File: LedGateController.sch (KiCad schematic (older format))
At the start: 48 parts, among them J1 5050_OUT, J2 SWD, J3 GPIO, Q1 FS8205A, Q2 AO3400A, Q3 AO3400A, Q4 AO3400A, SW1 SW_SPST, SW2 BUTTON, U1 AP2127N-3.3, U2 MT3608, U3 DW01, U4 STM32F030F4Px

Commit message: Move to footprints
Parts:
- removed Q3, Q4: AO3400A, Package_TO_SOT_SMD:SOT-23, symbol MiscParts:AO3400A
- removed R11, R12, R13: 100, Resistor_SMD:R_0805_2012Metric_Pad1.15x1.40mm_HandSolder, symbol Device:R
- removed TP3: +3V3, TestPoint:TestPoint_THTPad_2.0x2.0mm_Drill1.0mm, symbol Connector:TestPoint
- removed TP4: +12V, TestPoint:TestPoint_THTPad_2.0x2.0mm_Drill1.0mm, symbol Connector:TestPoint
- removed TP7: NRST, TestPoint:TestPoint_THTPad_2.0x2.0mm_Drill1.0mm, symbol Connector:TestPoint
- removed U1: AP2127N-3.3, Package_TO_SOT_SMD:SOT-23, symbol Regulator_Linear:AP2127N-3.3
- added C12, C14: 100n, Capacitor_SMD:C_0805_2012Metric_Pad1.15x1.40mm_HandSolder, symbol Device:C
- added C13: 470u, Capacitor_SMD:CP_Elec_10x7.7, symbol Device:CP
- added Q3: AO3401A, Package_TO_SOT_SMD:SOT-23, symbol Transistor_FET:AO3401A
- added R6, R7: 100, Resistor_SMD:R_0805_2012Metric_Pad1.15x1.40mm_HandSolder, symbol Device:R
- added TP5: LED_DATA_3V3, TestPoint:TestPoint_THTPad_D2.0mm_Drill1.0mm, symbol Connector:TestPoint
- added TP6: LED_DATA_5V, TestPoint:TestPoint_THTPad_D2.0mm_Drill1.0mm, symbol Connector:TestPoint
- added U4: XC6206P332MR, Package_TO_SOT_SMD:SOT-23, symbol Regulator_Linear:XC6206PxxxMR
- added U5: PI4ULS5V201, Package_TO_SOT_SMD:SOT-23-6_Handsoldering, symbol MiscParts:PI4ULS5V201
- BT1: value 18650 -> LI_ON; Digikey Part (none) -> https://www.digikey.co.uk/product-detail/en/keystone-electr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
- C1: renamed from C9; value 100nF -> 100n; footprint (none) -> Capacitor_SMD:C_0805_2012Metric_Pad1.15x1.40mm_HandSolder; LCSC Part (none) -> https://lcsc.com/product-detail/Multilayer-Ceramic-Capacito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
- C10: renamed from C1; value 0.1uF -> 1u; LCSC Part (none) -> https://lcsc.com/product-detail/Multilayer-Ceramic-Capacito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
- C11: renamed from C4; value 0.1uF -> 1u; LCSC Part (none) -> https://lcsc.com/product-detail/Multilayer-Ceramic-Capacito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
- C2: value 22uF -> 22u; footprint (none) -> Capacitor_SMD:C_0805_2012Metric_Pad1.15x1.40mm_HandSolder; LCSC Part (none) -> https://lcsc.com/product-detail/Multilayer-Ceramic-Capacito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
- C3: renamed from C6; value 100nF -> 100n; footprint (none) -> Capacitor_SMD:C_0805_2012Metric_Pad1.15x1.40mm_HandSolder; LCSC Part (none) -> https://lcsc.com/product-detail/Multilayer-Ceramic-Capacito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
- C4: renamed from C10; value 100nF -> 100n; footprint (none) -> Capacitor_SMD:C_0805_2012Metric_Pad1.15x1.40mm_HandSolder; LCSC Part (none) -> https://lcsc.com/product-detail/Multilayer-Ceramic-Capacito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
- C5: renamed from C3; value 0.1uF -> 100n; LCSC Part (none) -> https://lcsc.com/product-detail/Multilayer-Ceramic-Capacito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
- C6: renamed from C11; value 4.7uF -> 4u7; footprint (none) -> Capacitor_SMD:C_0805_2012Metric_Pad1.15x1.40mm_HandSolder; LCSC Part (none) -> https://lcsc.com/product-detail/Multilayer-Ceramic-Capacito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
- C7: renamed from C12; value 1uF -> 1u; footprint (none) -> Capacitor_SMD:C_0805_2012Metric_Pad1.15x1.40mm_HandSolder
- C8: renamed from C13; value 10nF -> 10n; footprint (none) -> Capacitor_SMD:C_0805_2012Metric_Pad1.15x1.40mm_HandSolder; LCSC Part (none) -> https://lcsc.com/product-detail/Multilayer-Ceramic-Capacito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
- C9: renamed from C5; value 22uF -> 22u; footprint (none) -> Capacitor_SMD:C_0805_2012Metric_Pad1.15x1.40mm_HandSolder; LCSC Part (none) -> https://lcsc.com/product-detail/Multilayer-Ceramic-Capacito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
- D1: value D_Schottky -> SS22; footprint (none) -> Diode_SMD:D_SMA_Handsoldering; LCSC Part (none) -> https://lcsc.com/product-detail/Schottky-Barrier-Diodes-SBD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
- D2: footprint (none) -> LED_SMD:LED_0805_2012Metric_Pad1.12x1.40mm_HandSolder; LCSC Part (none) -> https://jlcpcb.com/parts/componentSearch?secondSortUuid=ac4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
- J1: renamed from J3; footprint (none) -> Connector_PinHeader_2.54mm:PinHeader_1x10_P2.54mm_Vertical
- J2: footprint (none) -> Connector_PinHeader_2.54mm:PinHeader_1x05_P2.54mm_Vertical; symbol Connector:Conn_01x04_Male -> Connector:Conn_01x05_Male
- J3: renamed from J1; value 5050_OUT -> LED_OUT; footprint (none) -> Connector_PinHeader_2.54mm:PinHeader_1x03_P2.54mm_Horizontal; symbol Connector:Conn_01x04_Male -> Connector:Conn_01x03_Male
- L1: value 22uH -> 22u; footprint (none) -> Inductor_SMD:L_10.4x10.4_H4.8; LCSC Part (none) -> https://lcsc.com/product-detail/Power-Inductors_TDG-TMAX-10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
- Q1: footprint SOP65P640X120-8N -> Package_SO:TSSOP-8_4.4x3mm_P0.65mm; LCSC Part (none) -> https://lcsc.com/product-detail/MOSFET_Fortune-Semicon-FS82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
- Q2: LCSC Part (none) -> https://lcsc.com/product-detail/MOSFET_UMW-Youtai-Semicondu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
- R1: value 100R -> 100; LCSC Part (none) -> https://lcsc.com/product-detail/Chip-Resistor-Surface-Mount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
- R10: renamed from R9; value 33k -> 100K; LCSC Part (none) -> https://lcsc.com/product-detail/Chip-Resistor-Surface-Mount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
- R2: renamed from R6; value 100k -> 100K; LCSC Part (none) -> https://lcsc.com/product-detail/Chip-Resistor-Surface-Mount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
- R3: renamed from R2; value 5.6k -> 15K; LCSC Part (none) -> https://lcsc.com/product-detail/Chip-Resistor-Surface-Mount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
- R4: renamed from R3; value 100k -> 110K; LCSC Part (none) -> https://lcsc.com/product-detail/Chip-Resistor-Surface-Mount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
- R5: renamed from R4; value 1kR -> 1K; LCSC Part (none) -> https://lcsc.com/product-detail/Chip-Resistor-Surface-Mount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
- R8: renamed from R5; value 330R -> 150; LCSC Part (none) -> https://lcsc.com/product-detail/Chip-Resistor-Surface-Mount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
- R9: renamed from R8; value 100k -> 50K; LCSC Part (none) -> https://lcsc.com/product-detail/Chip-Resistor-Surface-Mount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
- SW1: renamed from SW2; footprint (none) -> Button_Switch_THT:SW_PUSH_6mm; LCSC Part (none) -> https://lcsc.com/product-detail/Tactile-Switches_SHOU-HAN-T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
- SW2: renamed from SW1; value SW_SPST -> ON_OFF; footprint (none) -> Button_Switch_THT:SW_CuK_OS102011MA1QN1_SPDT_Angled; symbol Switch:SW_SPST -> Switch:SW_SPDT; LCSC Part (none) -> https://lcsc.com/product-detail/Toggle-Switches_C-K_OS10201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
- TP2: footprint TestPoint:TestPoint_THTPad_2.0x2.0mm_Drill1.0mm -> TestPoint:TestPoint_THTPad_D2.0mm_Drill1.0mm
- TP3: renamed from TP8; value 12V_FB -> 5V_FB; footprint TestPoint:TestPoint_THTPad_2.0x2.0mm_Drill1.0mm -> TestPoint:TestPoint_THTPad_D2.0mm_Drill1.0mm
- U1: renamed from U4; LCSC Part (none) -> https://lcsc.com/product-detail/Others_STMicroelectronics_S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
- U2: footprint SOT95P280X145-6N -> Package_TO_SOT_SMD:SOT-23-6_Handsoldering; LCSC Part (none) -> https://lcsc.com/product-detail/DC-DC-Converters_MT3608_C84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
- U3: footprint SOT95P280X135-6N -> Package_TO_SOT_SMD:SOT-23-6_Handsoldering; LCSC Part (none) -> https://lcsc.com/product-detail/MOSFET_DW01_C181096.html; Manufacturer_Name Slkor -> (none)
- renumbered TP6 to TP4, TP5 to TP7
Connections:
- net labels added: +5V, +BATT_SW, LED_DATA_3V3, LED_DATA_5V, LED_EN, NRST, PA6, PA7
- net labels removed: +12V, -BATT, B, G, PA2, PA9, R
- wire segments 138 -> 177
- no-connect marks 5 -> 4
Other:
- note added: "Battery Switch"
- note added: "LED Logic Shifter"
- note added: "LED Supply (5V)"
- note removed: "LED Supply (12V)"
- moved on the sheet: C1, C10, C11, C2, C3, C4, C5, C6, C7, C8, C9, D1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

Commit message: nearly done
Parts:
- J1: footprint Connector_PinHeader_2.54mm:PinHeader_1x10_P2.54mm_Vertical -> Connector_PinHeader_2.54mm:PinHeader_1x06_P2.54mm_Vertical; symbol Connector_Generic:Conn_01x10 -> Connector_Generic:Conn_01x06
- SW1: footprint Button_Switch_THT:SW_PUSH_6mm -> LedGateController:TS-1009B-04326; LCSC Part https://lcsc.com/product-detail/Tactile-Switches_SHOU-HAN-T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 -> https://lcsc.com/product-detail/Tactile-Switches_XUNPU-TS-1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
- SW2: footprint Button_Switch_THT:SW_CuK_OS102011MA1QN1_SPDT_Angled -> SamacSys_Parts:SK12D07VG4NSPA; LCSC Part https://lcsc.com/product-detail/Toggle-Switches_C-K_OS10201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 -> https://lcsc.com/product-detail/Toggle-Switches_SHOU-HAN-SK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
- TP1, TP2, TP3, TP4, TP5, TP6, TP7: footprint TestPoint:TestPoint_THTPad_D2.0mm_Drill1.0mm -> TestPoint:TestPoint_THTPad_D1.5mm_Drill0.7mm
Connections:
- net labels added: PA1, PA2
- net labels removed: PA10, PA3, PA4, PA7
- wire segments 177 -> 173
- no-connect marks 4 -> 6
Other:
- moved on the sheet: C2, C9, D1, L1, R3, R4, TP3, U2

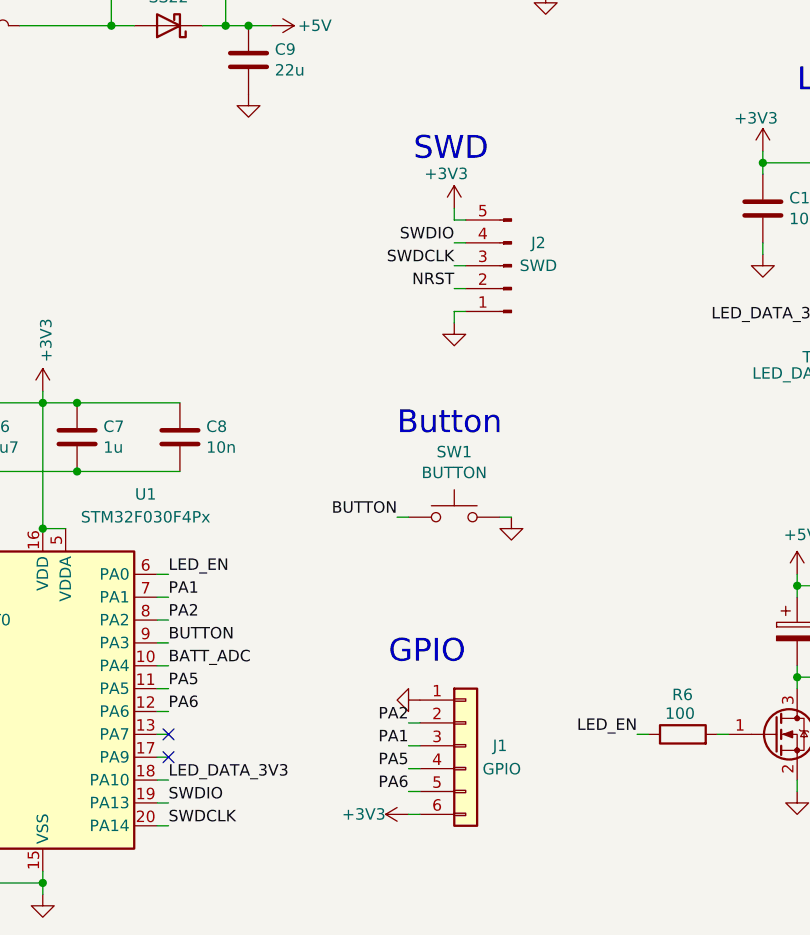
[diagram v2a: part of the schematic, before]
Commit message: Rev. 1 nearly ready!
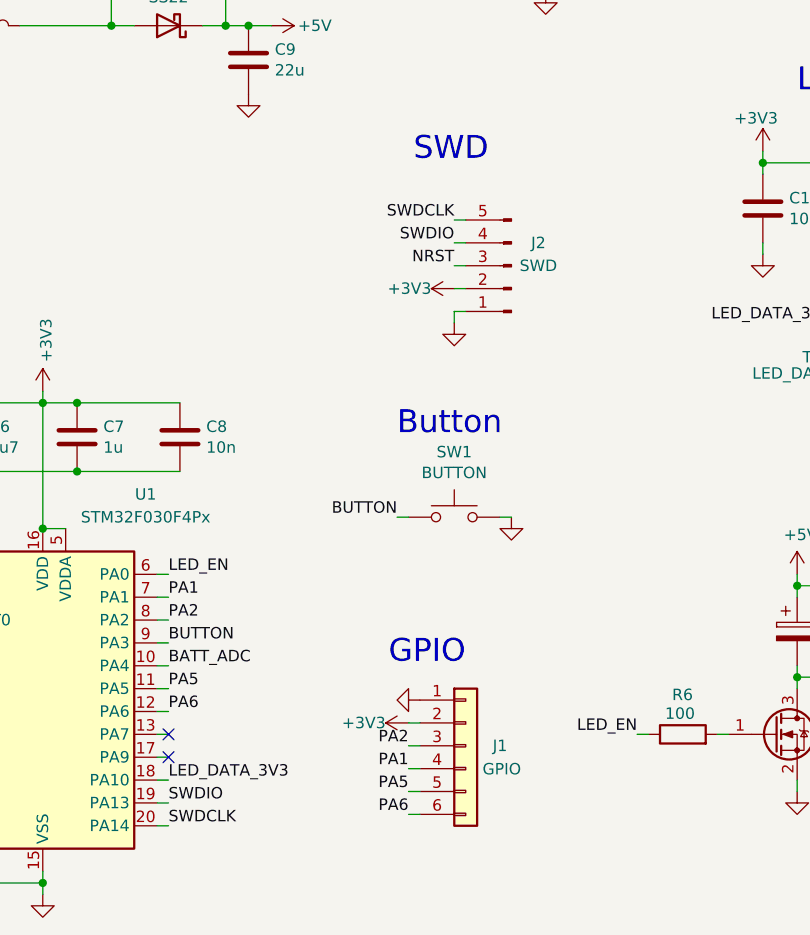
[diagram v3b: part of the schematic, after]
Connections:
- net +3V3: now also J1.2 (Pin_2), J2.2 (Pin_2); no longer J1.6 (Pin_6), J2.5 (Pin_5)
- net NRST: now also J2.3 (Pin_3); no longer J2.2 (Pin_2)
- net PA1: now also J1.4 (Pin_4); no longer J1.3 (Pin_3)
- net PA2: now also J1.3 (Pin_3); no longer J1.2 (Pin_2)
- net PA5: now also J1.5 (Pin_5); no longer J1.4 (Pin_4)
- net PA6: now also J1.6 (Pin_6); no longer J1.5 (Pin_5)
- net SWDCLK: now also J2.5 (Pin_5); no longer J2.3 (Pin_3)
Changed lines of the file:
@@
 L power:+3V3 #PWR015
 U 1 1 5F189137
-P 3900 4500
-F 0 "#PWR015" H 3900 4350 50  0001 C CNN
-F 1 "+3V3" H 3769 4652 50  0000 L CNN
-F 2 "" H 3900 4500 50  0001 C CNN
-F 3 "" H 3900 4500 50  0001 C CNN
-	1    3900 4500
-	1    0    0    -1
+P 3900 4850
+F 0 "#PWR015" H 3900 4700 50  0001 C CNN
+F 1 "+3V3" V 3900 4950 50  0000 L CNN
+F 2 "" H 3900 4850 50  0001 C CNN
+F 3 "" H 3900 4850 50  0001 C CNN
+	1    3900 4850
+	0    -1   -1   0
 $EndComp
 Wire Wire Line
@@
 	4300 3500 4300 3550
 Wire Wire Line
-	3900 4550 3900 4500
-Wire Wire Line
 	3900 5000 3900 4950
 Wire Wire Line
@@
 	0    -1   -1   0
 $EndComp
-Text Label 3700 6850 2    50   ~ 0
+Text Label 3700 6950 2    50   ~ 0
 PA1
-Text Label 3700 7050 2    50   ~ 0
+Text Label 3700 7150 2    50   ~ 0
 PA6
 Wire Wire Line
@@
 Wire Wire Line
 	3700 7150 3750 7150
-Text Label 3700 6950 2    50   ~ 0
+Text Label 3700 7050 2    50   ~ 0
 PA5
-Text Label 3700 6750 2    50   ~ 0
+Text Label 3700 6850 2    50   ~ 0
 PA2
 $Comp
@@
 	0    1    1    0
 $EndComp
+NoConn ~ 2650 6800
+NoConn ~ 2650 6900
 $Comp
 L power:+3V3 #PWR011
 U 1 1 5F2CFCAD
-P 3700 7150
-F 0 "#PWR011" H 3700 7000 50  0001 C CNN
-F 1 "+3V3" V 3700 7250 50  0000 L CNN
-F 2 "" H 3700 7150 50  0001 C CNN
-F 3 "" H 3700 7150 50  0001 C CNN
-	1    3700 7150
+P 3700 6750
+F 0 "#PWR011" H 3700 6600 50  0001 C CNN
+F 1 "+3V3" V 3700 6850 50  0000 L CNN
+F 2 "" H 3700 6750 50  0001 C CNN
+F 3 "" H 3700 6750 50  0001 C CNN
+	1    3700 6750
 	0    -1   -1   0
 $EndComp
-NoConn ~ 2650 6800
-NoConn ~ 2650 6900
+Text Label 3900 4750 2    50   ~ 0
+NRST
+Text Label 3900 4550 2    50   ~ 0
+SWDCLK
 Text Label 3900 4650 2    50   ~ 0
 SWDIO
-Text Label 3900 4750 2    50   ~ 0
-SWDCLK
-Text Label 3900 4850 2    50   ~ 0
-NRST
 $EndSCHEMATC

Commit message: Fix inductor schematic
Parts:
- L1: footprint Inductor_SMD:L_10.4x10.4_H4.8 -> LedGateController:YT1040-220M
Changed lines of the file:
@@
 F 0 "L1" V 2040 3700 50  0000 C CNN
 F 1 "22u" V 1949 3700 50  0000 C CNN
-F 2 "Inductor_SMD:L_10.4x10.4_H4.8" H 1850 3700 50  0001 C CNN
+F 2 "LedGateController:YT1040-220M" V 1750 3650 50  0001 C CNN
 F 3 "~" H 1850 3700 50  0001 C CNN
 F 4 "https://lcsc.com/product-detail/Power-Inductors_TDG-TMAX-1040-220-M_C429809.html" V 1850 3700 50  0001 C CNN "LCSC Part"
